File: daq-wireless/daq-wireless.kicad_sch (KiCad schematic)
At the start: 2 parts

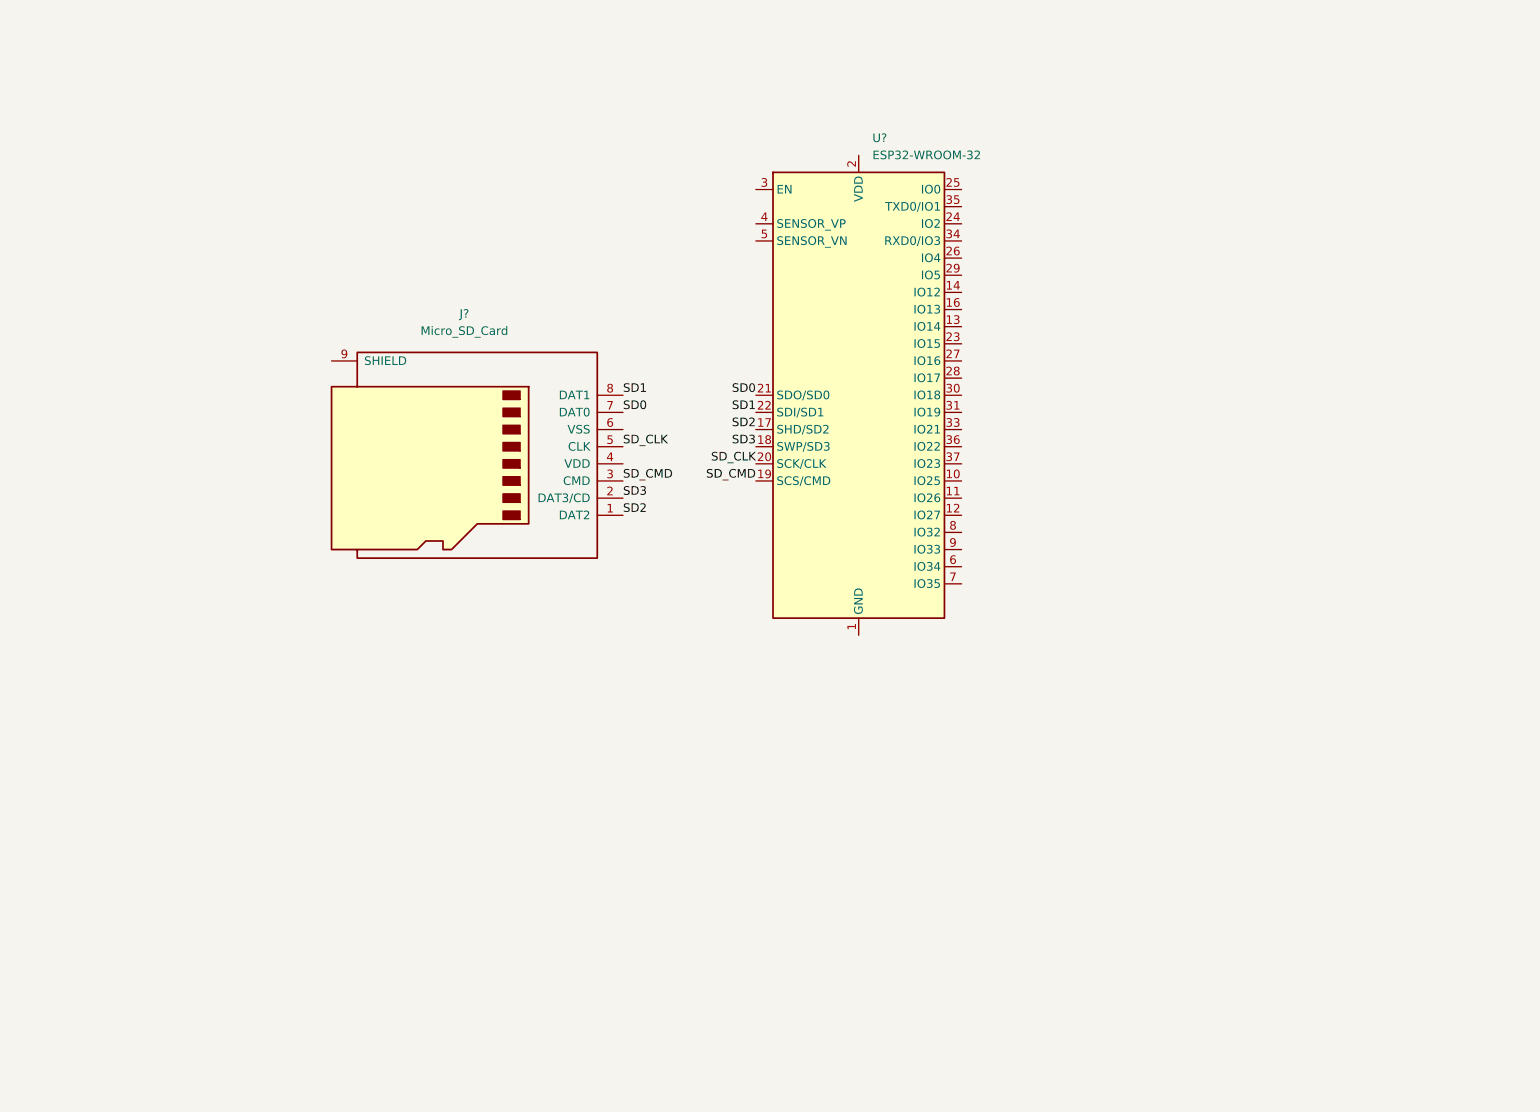
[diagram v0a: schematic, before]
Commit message: Easter eggs
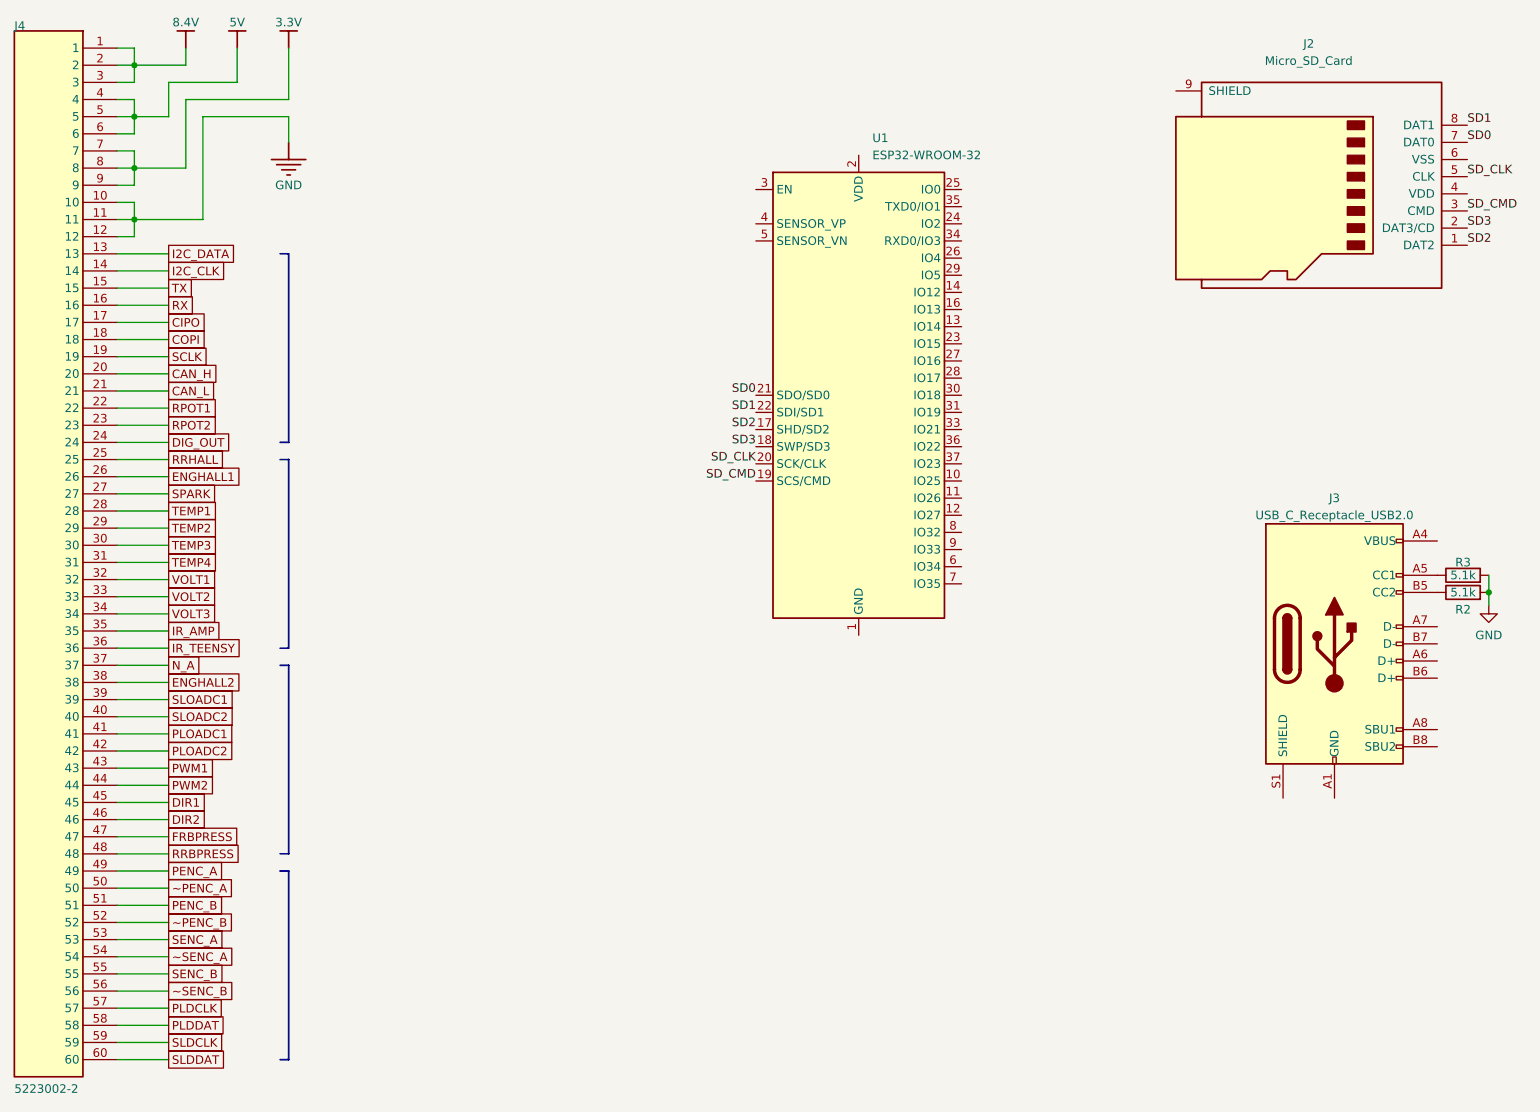
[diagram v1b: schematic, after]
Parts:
- added J3: USB_C_Receptacle_USB2.0, symbol Connector:USB_C_Receptacle_USB2.0
- added J4: 5223002-2, !footprints:52230042, symbol semiactive-altium-import:0_mirrored_5223002-2
- added R2, R3: 5.1k, symbol Device:R
- J2: renamed from J?; footprint (none) -> Connector_Card:microSD_HC_Hirose_DM3AT-SF-PEJM5
- gave numbers to parts that had none: 1
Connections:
- new net: J3.A1 (GND), J3.A12 (GND), J3.B1 (GND), J3.B12 (GND)
- new net: J3.A4 (VBUS), J3.A9 (VBUS), J3.B4 (VBUS), J3.B9 (VBUS)
- new net: J3.A5 (CC1), R3.1
- new net: J3.B5 (CC2), R2.1
- new net 3.3V: J4.7, J4.8, J4.9
- new net 5V: J4.4, J4.5, J4.6
- new net 8.4V: J4.1, J4.2, J4.3
- new net CAN_H: J4.20
- new net CAN_L: J4.21
- new net CIPO: J4.17
- new net COPI: J4.18
- new net DIG_OUT: J4.24
- new net DIR1: J4.45
- new net DIR2: J4.46
- new net ENGHALL1: J4.26
- new net ENGHALL2: J4.38
- new net FRBPRESS: J4.47
- new net GND: J4.10, J4.11, J4.12, R2.2, R3.2
- new net I2C_CLK: J4.14
- new net I2C_DATA: J4.13
- new net IR_AMP: J4.35
- new net IR_TEENSY: J4.36
- new net N_A: J4.37
- new net PENC_A: J4.49
- new net PENC_B: J4.51
- new net PLDCLK: J4.57
- new net PLDDAT: J4.58
- new net PLOADC1: J4.41
- new net PLOADC2: J4.42
- new net PWM1: J4.43
- new net PWM2: J4.44
- new net RPOT1: J4.22
- new net RPOT2: J4.23
- new net RRBPRESS: J4.48
- new net RRHALL: J4.25
- new net RX: J4.16
- new net SCLK: J4.19
- new net SENC_A: J4.53
- new net SENC_B: J4.55
- new net SLDCLK: J4.59
- new net SLDDAT: J4.60
- new net SLOADC1: J4.39
- new net SLOADC2: J4.40
- new net SPARK: J4.27
- new net TEMP1: J4.28
- new net TEMP2: J4.29
- new net TEMP3: J4.30
- new net TEMP4: J4.31
- new net TX: J4.15
- new net VOLT1: J4.32
- new net VOLT2: J4.33
- new net VOLT3: J4.34
- new net ~PENC_A: J4.50
- new net ~PENC_B: J4.52
- new net ~SENC_A: J4.54
- new net ~SENC_B: J4.56
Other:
- moved on the sheet: J2
